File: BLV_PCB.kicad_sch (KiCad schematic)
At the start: 10 parts, among them J1 JST-PH, J2 JST-PH, J3 JST-PH, J4 duPont, J5 duPont, J6 duPont

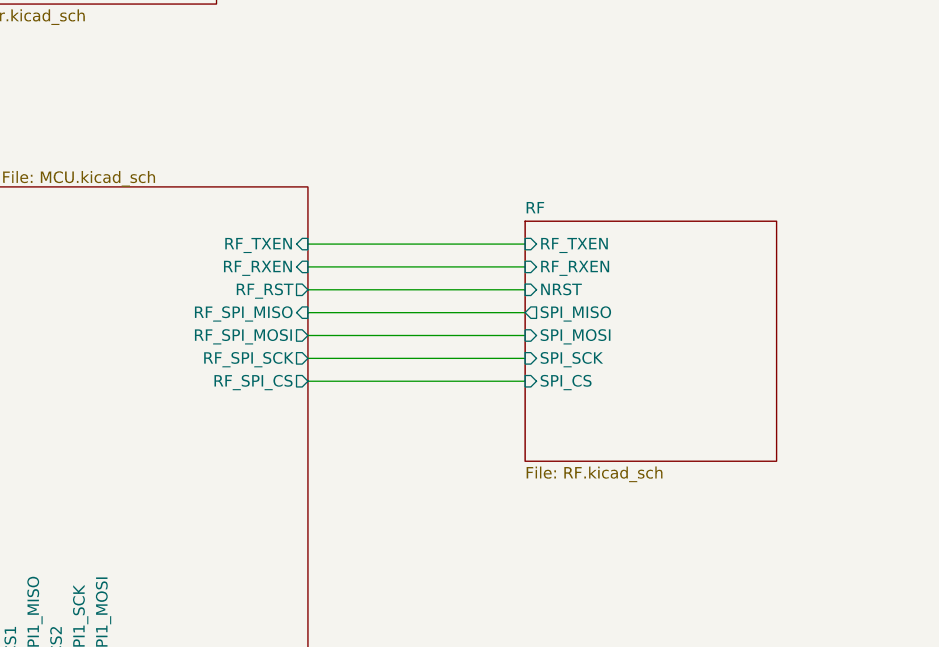
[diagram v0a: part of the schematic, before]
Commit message: v1.0.1 - RF Fix
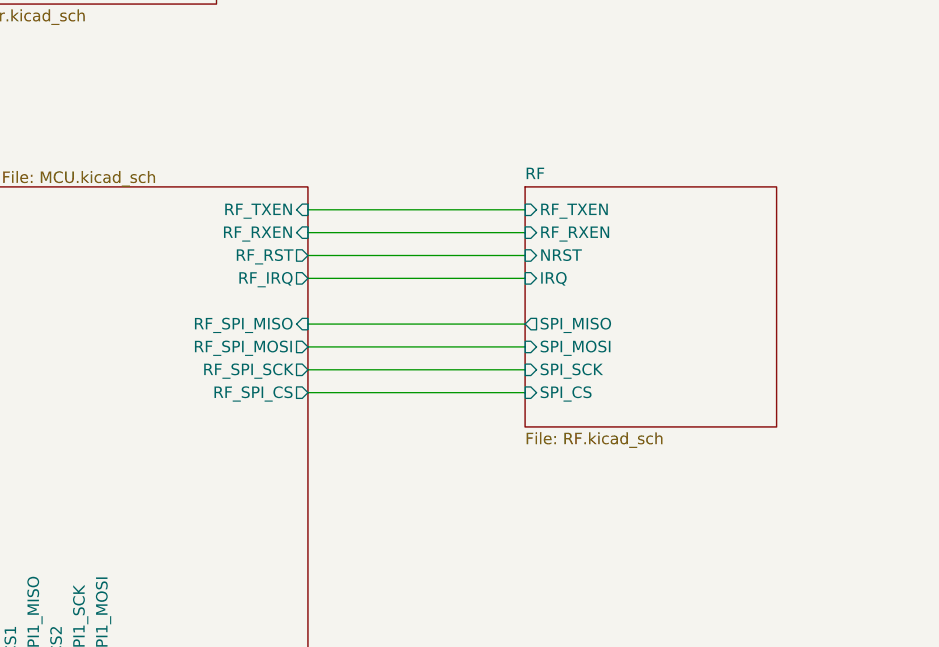
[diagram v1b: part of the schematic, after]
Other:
- sheet MCU ports: added RF_IRQ; removed none
- sheet RF ports: added IRQ; removed none
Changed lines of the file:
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@@
+	(wire
+		(pts
+			(xy 191.77 81.28) (xy 215.9 81.28)
+		)
+		(stroke
+			(width 0)
+			(type default)
+		)
+	)
 	(wire
 		(pts
@@
 	(wire
 		(pts
+			(xy 191.77 91.44) (xy 215.9 91.44)
+		)
+		(stroke
+			(width 0)
+			(type default)
+		)
+	)
+	(wire
+		(pts
 			(xy 81.28 81.28) (xy 121.92 81.28)
 		)
@@
 	(wire
 		(pts
-			(xy 191.77 92.71) (xy 215.9 92.71)
-		)
-		(stroke
-			(width 0)
-			(type default)
-		)
-	)
-	(wire
-		(pts
 			(xy 81.28 104.14) (xy 119.38 104.14)
 		)
@@
 	(wire
 		(pts
-			(xy 191.77 90.17) (xy 215.9 90.17)
-		)
-		(stroke
-			(width 0)
-			(type default)
-		)
-	)
-	(wire
-		(pts
 			(xy 93.98 121.92) (xy 95.25 121.92)
 		)
@@
 	(wire
 		(pts
+			(xy 191.77 83.82) (xy 215.9 83.82)
+		)
+		(stroke
+			(width 0)
+			(type default)
+		)
+	)
+	(wire
+		(pts
 			(xy 121.92 106.68) (xy 139.7 106.68)
 		)
@@
 	(wire
 		(pts
-			(xy 191.77 95.25) (xy 215.9 95.25)
-		)
-		(stroke
-			(width 0)
-			(type default)
-		)
-	)
-	(wire
-		(pts
-			(xy 191.77 87.63) (xy 215.9 87.63)
-		)
-		(stroke
-			(width 0)
-			(type default)
-		)
-	)
-	(wire
-		(pts
 			(xy 163.83 134.62) (xy 163.83 165.1)
 		)
@@
 	(wire
 		(pts
+			(xy 191.77 93.98) (xy 215.9 93.98)
+		)
+		(stroke
+			(width 0)
+			(type default)
+		)
+	)
+	(wire
+		(pts
+			(xy 191.77 99.06) (xy 215.9 99.06)
+		)
+		(stroke
+			(width 0)
+			(type default)
+		)
+	)
+	(wire
+		(pts
 			(xy 81.28 106.68) (xy 121.92 106.68)
 		)
@@
 	(wire
 		(pts
-			(xy 191.77 85.09) (xy 215.9 85.09)
-		)
-		(stroke
-			(width 0)
-			(type default)
-		)
-	)
-	(wire
-		(pts
 			(xy 166.37 134.62) (xy 166.37 165.1)
 		)
@@
 	(wire
 		(pts
+			(xy 191.77 78.74) (xy 215.9 78.74)
+		)
+		(stroke
+			(width 0)
+			(type default)
+		)
+	)
+	(wire
+		(pts
 			(xy 93.98 96.52) (xy 95.25 96.52)
 		)
@@
 	(wire
 		(pts
-			(xy 191.77 82.55) (xy 215.9 82.55)
-		)
-		(stroke
-			(width 0)
-			(type default)
-		)
-	)
-	(wire
-		(pts
 			(xy 81.28 132.08) (xy 121.92 132.08)
 		)
@@
 	(wire
 		(pts
+			(xy 191.77 86.36) (xy 215.9 86.36)
+		)
+		(stroke
+			(width 0)
+			(type default)
+		)
+	)
+	(wire
+		(pts
 			(xy 121.92 81.28) (xy 121.92 93.98)
 		)
@@
 	(wire
 		(pts
-			(xy 191.77 97.79) (xy 215.9 97.79)
-		)
-		(stroke
-			(width 0)
-			(type default)
-		)
-	)
-	(wire
-		(pts
 			(xy 119.38 104.14) (xy 139.7 104.14)
+		)
+		(stroke
+			(width 0)
+			(type default)
+		)
+	)
+	(wire
+		(pts
+			(xy 191.77 96.52) (xy 215.9 96.52)
 		)
 		(stroke
@@
 		)
 		(pin "RF_SPI_CS" output
-			(at 191.77 97.79 0)
+			(at 191.77 99.06 0)
 			(effects
 				(font
@@
 		)
 		(pin "RF_SPI_MISO" input
-			(at 191.77 90.17 0)
+			(at 191.77 91.44 0)
 			(effects
 				(font
@@
 		)
 		(pin "RF_SPI_MOSI" output
-			(at 191.77 92.71 0)
+			(at 191.77 93.98 0)
 			(effects
 				(font
@@
 		)
 		(pin "RF_SPI_SCK" output
-			(at 191.77 95.25 0)
+			(at 191.77 96.52 0)
 			(effects
 				(font
@@
 		)
 		(pin "RF_RST" output
-			(at 191.77 87.63 0)
+			(at 191.77 83.82 0)
 			(effects
 				(font
@@
 		)
 		(pin "RF_RXEN" input
-			(at 191.77 85.09 0)
+			(at 191.77 81.28 0)
 			(effects
 				(font
@@
 		)
 		(pin "RF_TXEN" input
-			(at 191.77 82.55 0)
+			(at 191.77 78.74 0)
+			(effects
+				(font
+					(size 1.27 1.27)
+				)
+				(justify right)
+			)
+		)
+		(pin "RF_IRQ" output
+			(at 191.77 86.36 0)
 			(effects
 				(font
@@
 	)
 	(sheet
-		(at 215.9 80.01)
+		(at 215.9 76.2)
 		(size 27.94 26.67)
 		(exclude_from_sim no)
@@
 		)
 		(property "Sheetname" "RF"
-			(at 215.9 79.2984 0)
+			(at 215.9 75.4884 0)
 			(effects
 				(font
@@
 		)
 		(property "Sheetfile" "RF.kicad_sch"
-			(at 215.9 107.2646 0)
+			(at 215.9 103.4546 0)
 			(effects
 				(font
@@
 		)
 		(property "Field2" ""
-			(at 215.9 80.01 0)
+			(at 215.9 76.2 0)
 			(effects
 				(font
@@
 		)
 		(pin "NRST" input
-			(at 215.9 87.63 180)
+			(at 215.9 83.82 180)
 			(effects
 				(font
@@
 		)
 		(pin "SPI_CS" input
-			(at 215.9 97.79 180)
+			(at 215.9 99.06 180)
 			(effects
 				(font
@@
 		)
 		(pin "SPI_MISO" output
-			(at 215.9 90.17 180)
+			(at 215.9 91.44 180)
 			(effects
 				(font
@@
 		)
 		(pin "SPI_MOSI" input
-			(at 215.9 92.71 180)
+			(at 215.9 93.98 180)
 			(effects
 				(font
@@
 		)
 		(pin "SPI_SCK" input
-			(at 215.9 95.25 180)
+			(at 215.9 96.52 180)
 			(effects
 				(font
@@
 		)
 		(pin "RF_RXEN" input
-			(at 215.9 85.09 180)
+			(at 215.9 81.28 180)
 			(effects
 				(font
@@
 		)
 		(pin "RF_TXEN" input
-			(at 215.9 82.55 180)
-			(effects
-				(font
+			(at 215.9 78.74 180)
+			(effects
+				(font
+					(size 1.27 1.27)
+				)
+				(justify left)
+			)
+		)
+		(pin "IRQ" input
+			(at 215.9 86.36 180)
+			(effects
+				(font
